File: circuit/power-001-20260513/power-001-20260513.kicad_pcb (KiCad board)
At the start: 4 copper layers, 68.4 x 46.4 mm, 51 parts, among them J1 VIN, J2 +5V_{Line}, J3 Power, J4 Logic, J5 Sub_{Power}, J6 Sub_{Signal}, J7 ICSP_{PIC12F683}, J8 ESC, Q1 BSS138, Q2 PMOS, SW1 SW_SPDT, SW2 SW_SPDT, SW3 SW_SPDT, SW4 Locker_SW, U1 OKL-T/6-W12N-C, U2 OKL-T/6-W12N-C, U3 AZ1084-3.3, U5 PIC12F683-xSN, U6 LM1117MP-3.3

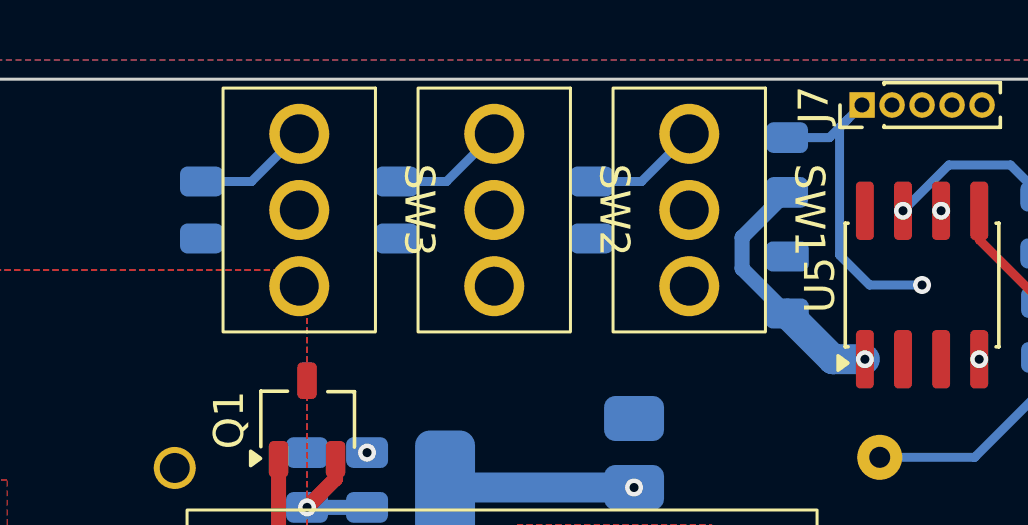
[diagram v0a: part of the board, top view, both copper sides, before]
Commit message: Update 電源基板の寸法変更を確認
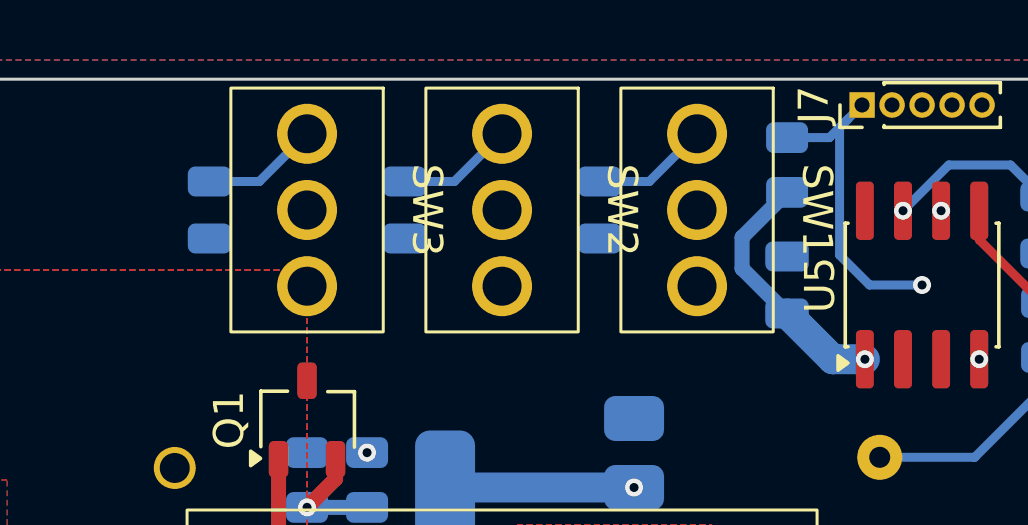
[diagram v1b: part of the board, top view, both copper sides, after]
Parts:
- moved C2 0.26 mm to (3.25, -17.5)
- moved C3 0.26 mm to (-3.25, -17.5)
- moved SW2 0.26 mm to (0.00, -17.5)
- moved C4 0.26 mm to (-9.75, -17.5)
- moved SW1 0.26 mm to (6.50, -17.5)
- moved SW3 0.26 mm to (-6.50, -17.5)
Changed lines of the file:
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@@
 	(footprint "@Thrive_footprint_power:2MS1-T1-B4-M2-Q-E"
 		(layer "F.Cu")
-		(at 6.239696 -17.499998 -90)
+		(at 6.5 -17.5 -90)
 		(property "Reference" "SW1"
 			(at 0 -4 270)
@@
 	(footprint "@Thrive_footprint_power:2MS1-T1-B4-M2-Q-E"
 		(layer "F.Cu")
-		(at -6.760304 -17.499998 -90)
+		(at -6.5 -17.5 -90)
 		(property "Reference" "SW3"
 			(at 0 -4 270)
@@
 	(footprint "@Thrive_footprint_power:2MS1-T1-B4-M2-Q-E"
 		(layer "F.Cu")
-		(at -0.260304 -17.499998 -90)
+		(at 0 -17.5 -90)
 		(property "Reference" "SW2"
 			(at 0 -4 270)
@@
 	(footprint "Capacitor_SMD:C_0805_2012Metric"
 		(layer "B.Cu")
-		(at -10.010304 -17.499998 -90)
+		(at -9.75 -17.5 -90)
 		(descr "Capacitor SMD 0805 (2012 Metric), square (rectangular) end terminal, IPC-7351 nominal, (Body size source: IPC-SM-782 page 76, https://www.pcb-3d.com/wordpress/wp-content/uploads/ipc-sm-782a_amendment_1_and_2.pdf, https://docs.google.com/spreadsheets/d/1BsfQQcO9C6DZCsRaXUlFlo91Tg2WpOkGARC1WS5S8t0/edit?usp=sharing)")
 		(tags "capacitor")
@@
 	(footprint "Capacitor_SMD:C_0805_2012Metric"
 		(layer "B.Cu")
-		(at -3.510304 -17.499998 -90)
+		(at -3.25 -17.5 -90)
 		(descr "Capacitor SMD 0805 (2012 Metric), square (rectangular) end terminal, IPC-7351 nominal, (Body size source: IPC-SM-782 page 76, https://www.pcb-3d.com/wordpress/wp-content/uploads/ipc-sm-782a_amendment_1_and_2.pdf, https://docs.google.com/spreadsheets/d/1BsfQQcO9C6DZCsRaXUlFlo91Tg2WpOkGARC1WS5S8t0/edit?usp=sharing)")
 		(tags "capacitor")
@@
 	(footprint "Capacitor_SMD:C_0805_2012Metric"
 		(layer "B.Cu")
-		(at 2.989696 -17.499998 -90)
+		(at 3.25 -17.5 -90)
 		(descr "Capacitor SMD 0805 (2012 Metric), square (rectangular) end terminal, IPC-7351 nominal, (Body size source: IPC-SM-782 page 76, https://www.pcb-3d.com/wordpress/wp-content/uploads/ipc-sm-782a_amendment_1_and_2.pdf, https://docs.google.com/spreadsheets/d/1BsfQQcO9C6DZCsRaXUlFlo91Tg2WpOkGARC1WS5S8t0/edit?usp=sharing)")
 		(tags "capacitor")
@@
 	)
 	(segment
-		(start 4.649695 -18.449997)
-		(end 2.989696 -18.449997)
+		(start 6.5 -20.04)
+		(end 4.909997 -18.449997)
 		(width 0.3)
 		(layer "B.Cu")
@@
 	)
 	(segment
-		(start 6.239696 -20.039998)
-		(end 4.649695 -18.449997)
+		(start 3.250002 -18.449997)
+		(end 3.25 -18.449999)
 		(width 0.3)
 		(layer "B.Cu")
@@
 	)
 	(segment
-		(start -32.400772 -13.109998)
-		(end 2.609998 -13.109998)
+		(start 4.909997 -18.449997)
+		(end 3.250002 -18.449997)
 		(width 0.3)
-		(layer "In2.Cu")
+		(layer "B.Cu")
 		(net "SW_TGL_1")
 	)
 	(segment
-		(start 2.609998 -13.109998)
-		(end 4.5 -15)
+		(start 4.75 -18.29)
+		(end 6.5 -20.04)
 		(width 0.3)
 		(layer "In2.Cu")
@@
 	)
 	(segment
-		(start 4.5 -15)
-		(end 4.5 -18.300302)
+		(start 4.75 -15.25)
+		(end 4.75 -18.29)
 		(width 0.3)
 		(layer "In2.Cu")
@@
 	)
 	(segment
-		(start 4.5 -18.300302)
-		(end 6.239696 -20.039998)
+		(start -32.400772 -13.109998)
+		(end 2.609998 -13.109998)
+		(width 0.3)
+		(layer "In2.Cu")
+		(net "SW_TGL_1")
+	)
+	(segment
+		(start 2.609998 -13.109998)
+		(end 4.75 -15.25)
 		(width 0.3)
 		(layer "In2.Cu")
@@
 	)
 	(segment
-		(start 11.025001 -12.525)
-		(end 12.095 -12.525)
-		(width 1)
+		(start 9.5 -18.0875)
+		(end 8 -16.5875)
+		(width 0.5)
 		(layer "B.Cu")
 		(net "+3.3VA")
 	)
 	(segment
-		(start 4.399999 -8.25)
-		(end -1.899999 -8.25)
+		(start 11.025001 -12.525)
+		(end 12.095 -12.525)
 		(width 1)
 		(layer "B.Cu")
@@
 	)
 	(segment
-		(start 9.5 -18.0875)
-		(end 8 -16.5875)
-		(width 0.5)
-		(layer "B.Cu")
-		(net "+3.3VA")
-	)
-	(segment
-		(start 9.5 -14.050001)
-		(end 11.025001 -12.525)
+		(start 4.399999 -8.25)
+		(end -1.899999 -8.25)
 		(width 1)
 		(layer "B.Cu")
@@
 	)
 	(segment
+		(start 9.5 -14.050001)
+		(end 11.025001 -12.525)
+		(width 1)
+		(layer "B.Cu")
+		(net "+3.3VA")
+	)
+	(segment
 		(start 11.25 -13.37)
 		(end 12.095 -12.525)
@@
 	)
 	(segment
-		(start -8.350305 -18.449997)
-		(end -10.010304 -18.449997)
+		(start -6.5 -20.04)
+		(end -8.090003 -18.449997)
+		(width 0.3)
+		(layer "B.Cu")
+		(net "SW_TGL_3")
+	)
+	(segment
+		(start -9.749998 -18.449997)
+		(end -9.75 -18.449999)
 		(width 0.3)
 		(layer "B.Cu")
@@
 	)
 	(segment
-		(start -6.760304 -20.039998)
-		(end -8.350305 -18.449997)
+		(start -8.090003 -18.449997)
+		(end -9.749998 -18.449997)
 		(width 0.3)
 		(layer "B.Cu")
@@
 	)
 	(segment
-		(start -6.760304 -20.039998)
-		(end -12.690304 -14.109998)
+		(start -6.5 -20.04)
+		(end -12.430002 -14.109998)
 		(width 0.3)
 		(layer "In2.Cu")
@@
 	)
 	(segment
-		(start -12.690304 -14.109998)
+		(start -12.430002 -14.109998)
 		(end -36.480772 -14.109998)
 		(width 0.3)
@@
 	)
 	(segment
-		(start -0.260304 -20.039998)
-		(end -1.850305 -18.449997)
+		(start -3.25 -18.449999)
+		(end -3.250002 -18.449997)
 		(width 0.3)
 		(layer "B.Cu")
@@
 	)
 	(segment
-		(start -1.850305 -18.449997)
-		(end -3.510304 -18.449997)
+		(start 0 -20.04)
+		(end -1.590001 -18.449999)
 		(width 0.3)
 		(layer "B.Cu")
@@
 	)
 	(segment
-		(start -34.440772 -13.609998)
-		(end -3.390002 -13.609998)
+		(start -1.590001 -18.449999)
+		(end -3.25 -18.449999)
+		(width 0.3)
+		(layer "B.Cu")
+		(net "SW_TGL_2")
+	)
+	(segment
+		(start -1.75 -18.29)
+		(end 0 -20.04)
 		(width 0.3)
 		(layer "In2.Cu")
@@
 	)
 	(segment
-		(start -2 -15)
-		(end -2 -18.300302)
+		(start -34.440772 -13.609998)
+		(end -3.390002 -13.609998)
 		(width 0.3)
 		(layer "In2.Cu")
@@
 	)
 	(segment
-		(start -2 -18.300302)
-		(end -0.260304 -20.039998)
+		(start -3.390002 -13.609998)
+		(end -1.75 -15.25)
 		(width 0.3)
 		(layer "In2.Cu")
@@
 	)
 	(segment
-		(start -3.390002 -13.609998)
-		(end -2 -15)
+		(start -1.75 -15.25)
+		(end -1.75 -18.29)
 		(width 0.3)
 		(layer "In2.Cu")
